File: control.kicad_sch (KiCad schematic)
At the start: 10 parts, among them IC10 INA260AIPWR, IC15 RP2354A, IC16 TPS2121RUXR, IC17 TCAN1046AVDRQ1, Q7 BSZ067N06LS3_G, Y1 ABM8-272-T3

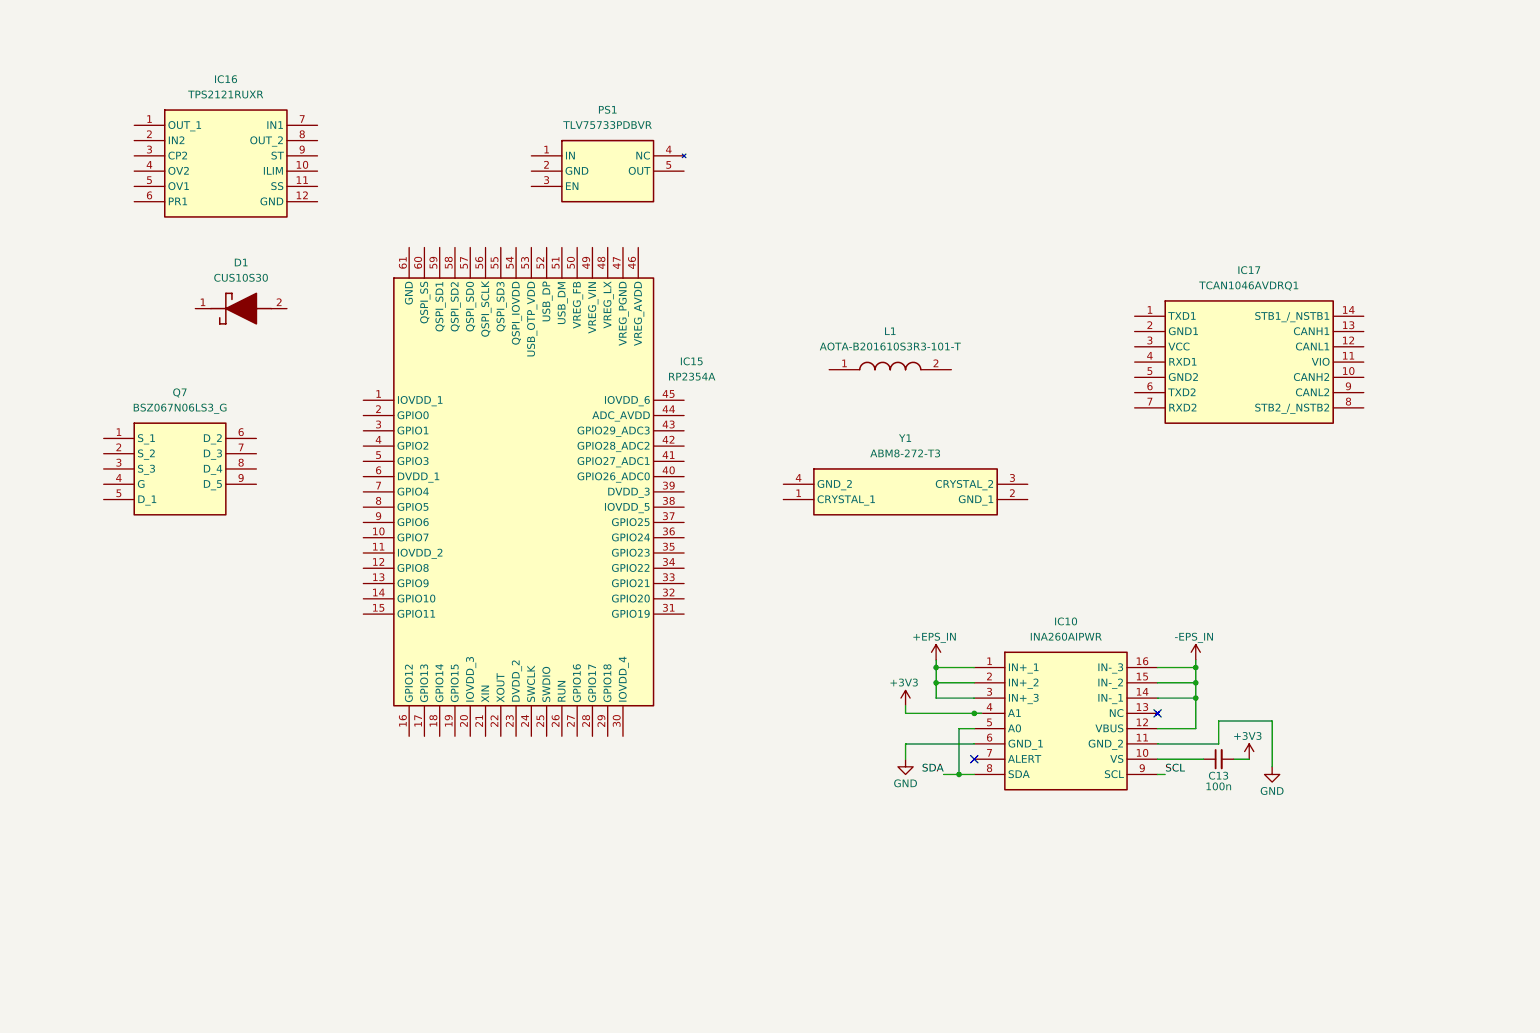
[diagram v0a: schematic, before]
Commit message: Test commit
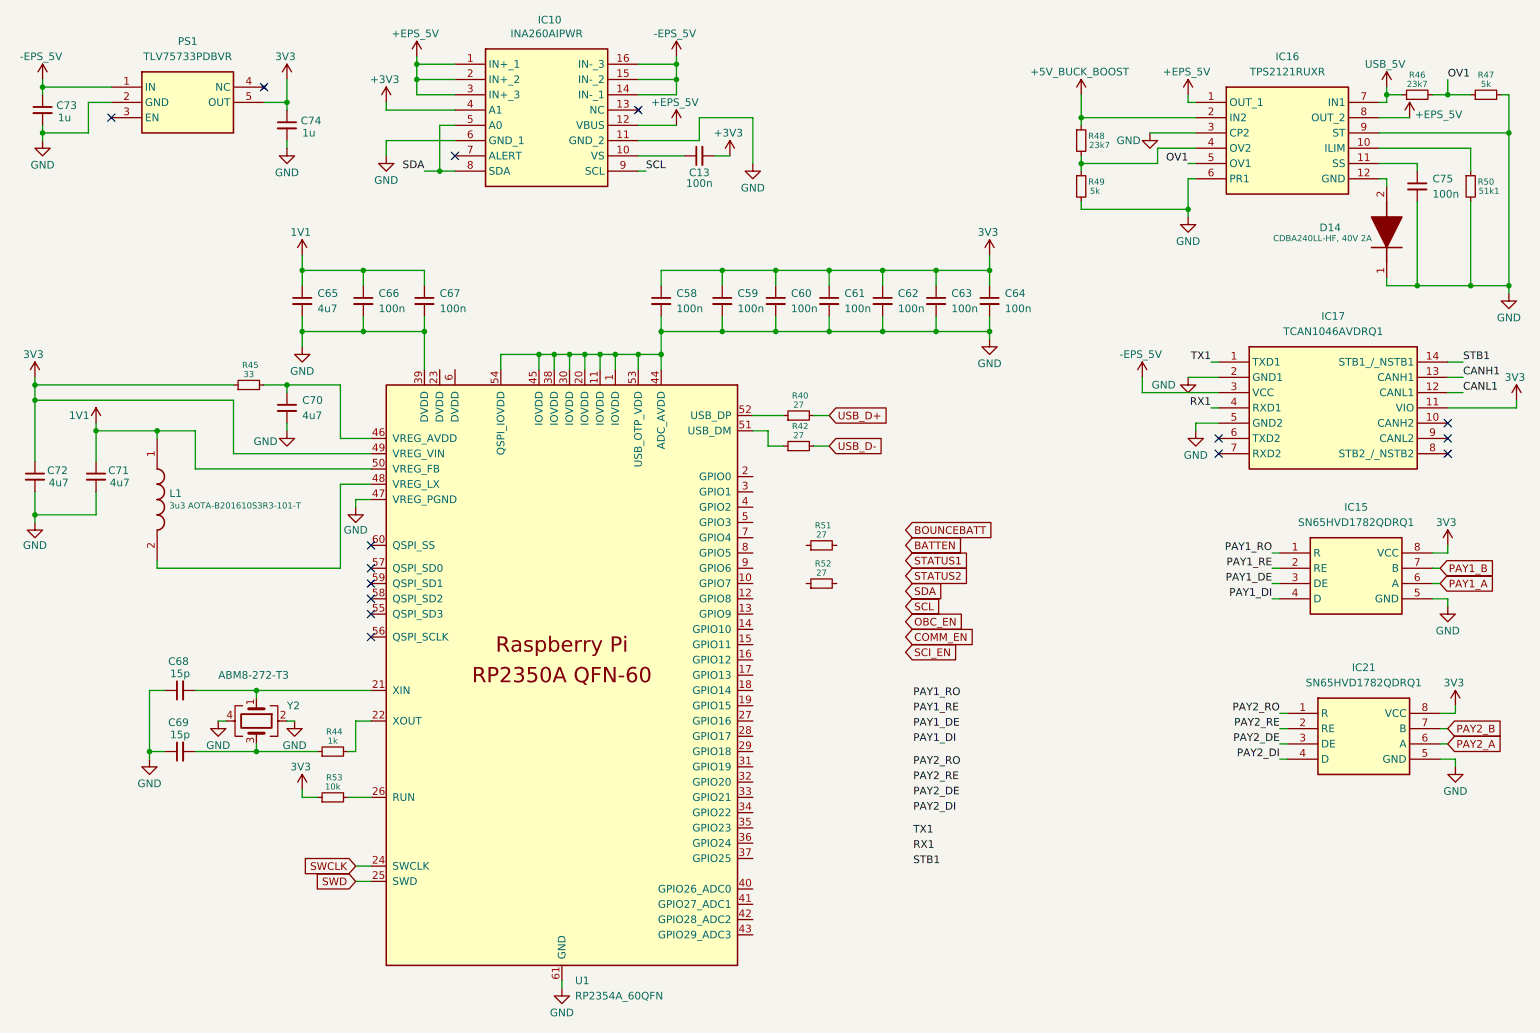
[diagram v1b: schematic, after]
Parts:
- removed D1: CUS10S30, CUS357H3F, symbol HEDGE2:CUS10S30
- removed IC15: RP2354A, QFN40P700X700X90-61N-D, symbol HEDGE2:RP2354A
- removed Q7: BSZ067N06LS3_G, BSZ067N06LS3G, symbol HEDGE2:BSZ067N06LS3_G
- removed Y1: ABM8-272-T3, ABM8272T3, symbol HEDGE2:ABM8-272-T3
- added C58, C59, C60, C61, C62, C63, C64, C66, C67, C75: 100n, symbol Device:C_Small
- added C65, C70, C71, C72: 4u7, symbol Device:C_Small
- added C68, C69: 15p, symbol Device:C_Small
- added C73, C74: 1u, symbol Device:C_Small
- added D14: CDBA240LL-HF, 40V 2A, DIOM5225X250N, symbol HEDGE2:CDBA240LL-HF
- added IC15, IC21: SN65HVD1782QDRQ1, SOIC127P600X175-8N, symbol HEDGE2:SN65HVD1782QDRQ1
- added R40, R42, R51, R52: 27, symbol Device:R_Small
- added R44: 1k, symbol Device:R_Small
- added R45: 33, symbol Device:R_Small
- added R46, R48: 23k7, symbol Device:R_Small
- added R47, R49: 5k, symbol Device:R_Small
- added R50: 51k1, symbol Device:R_Small
- added R53: 10k, symbol Device:R_Small
- added U1: RP2354A_60QFN, RP2354A_60QFN_minimal:RP2350-QFN-60-1EP_7x7_P0.4mm_EP3.4x3.4mm_ThermalVias, symbol MCU_RaspberryPi_RP2350:RP2350_60QFN
- added Y2: ABM8-272-T3, Crystal:Crystal_SMD_3225-4Pin_3.2x2.5mm, symbol Device:Crystal_GND24
- L1: value AOTA-B201610S3R3-101-T -> 3u3 AOTA-B201610S3R3-101-T
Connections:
- net +EPS_IN is gone; now on net +EPS_5V: IC10.1 (IN+_1), IC10.2 (IN+_2), IC10.3 (IN+_3)
- net GND: now also IC16.3 (CP2), IC16.6 (PR1), IC16.9 (ST), IC17.2 (GND1), IC17.5 (GND2), PS1.2 (GND), C58.2, C59.2, C60.2, C61.2, C62.2, C63.2, C64.2, C65.2, C66.2, C67.2, C68.1, C69.1, C70.2, C71.2, C72.2, C73.2, C74.2, C75.2, D14.1 (K), IC15.5 (GND), IC21.5 (GND), R47.2, R49.2, R50.2, U1.1 (IOVDD), U1.11 (IOVDD), U1.20 (IOVDD), U1.30 (IOVDD), U1.38 (IOVDD), U1.39 (DVDD), U1.44 (ADC_AVDD), U1.45 (IOVDD), U1.47 (VREG_PGND), U1.53 (USB_OTP_VDD), U1.54 (QSPI_IOVDD), U1.61 (GND), Y2.2, Y2.4
- net 1V1: now reaches L1.1
- net 1V1: now also C65.1, C66.1, C67.1, C71.1, U1.50 (VREG_FB)
- net at L1.2: now also U1.48 (VREG_LX)
- net +EPS_5V: now reaches IC16.1 (OUT_1)
- net +EPS_5V: now also IC10.12 (VBUS), IC16.8 (OUT_2)
- net at IC16.10 (ILIM): now also R50.1
- net at IC16.11 (SS): now also C75.1
- net at IC16.12 (GND): now also D14.2 (A)
- net +5V_BUCK_BOOST: now reaches IC16.2 (IN2)
- net +5V_BUCK_BOOST: now also R48.1
- net at IC16.4 (OV2): now also R48.2, R49.1
- net OV1: now reaches IC16.5 (OV1)
- net OV1: now also R46.2, R47.1
- net USB_5V: now reaches IC16.7 (IN1)
- net USB_5V: now also R46.1
- net -EPS_5V: now reaches PS1.1 (IN)
- net -EPS_5V: now also IC10.14 (IN-_1), IC10.15 (IN-_2), IC10.16 (IN-_3), IC17.3 (VCC), C73.1
- net 3V3: now reaches PS1.5 (OUT)
- net 3V3: now also IC17.11 (VIO), C58.1, C59.1, C60.1, C61.1, C62.1, C63.1, C64.1, C72.1, C74.1, IC15.8 (VCC), IC21.8 (VCC), R45.1, R53.1, U1.49 (VREG_VIN)
- net TX1: now reaches IC17.1 (TXD1)
- net CANL1: now reaches IC17.12 (CANL1)
- net CANH1: now reaches IC17.13 (CANH1)
- net STB1: now reaches IC17.14 (STB1_/_NSTB1)
- net RX1: now reaches IC17.4 (RXD1)
- removed net -EPS_IN: IC10.12 (VBUS), IC10.14 (IN-_1), IC10.15 (IN-_2), IC10.16 (IN-_3)
- new net: C68.2, U1.21 (XIN), Y2.1
- new net: C69.2, R44.1, Y2.3
- new net: R53.2, U1.26 (RUN)
- new net: R44.2, U1.22 (XOUT)
- new net: C70.1, R45.2, U1.46 (VREG_AVDD)
- new net: R42.1, U1.51 (USB_DM)
- new net: R40.1, U1.52 (USB_DP)
- new net PAY1_A: IC15.6 (A)
- new net PAY1_B: IC15.7 (B)
- new net PAY1_DE: IC15.3 (DE)
- new net PAY1_DI: IC15.4 (D)
- new net PAY1_RE: IC15.2 (RE)
- new net PAY1_RO: IC15.1 (R)
- new net PAY2_A: IC21.6 (A)
- new net PAY2_B: IC21.7 (B)
- new net PAY2_DE: IC21.3 (DE)
- new net PAY2_DI: IC21.4 (D)
- new net PAY2_RE: IC21.2 (RE)
- new net PAY2_RO: IC21.1 (R)
- new net SWCLK: U1.24 (SWCLK)
- new net SWD: U1.25 (SWD)
- new net USB_D+: R40.2
- new net USB_D-: R42.2
- no-connect marks 2 -> 15
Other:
- moved on the sheet: C13, IC10, IC16, IC17, L1, PS1
